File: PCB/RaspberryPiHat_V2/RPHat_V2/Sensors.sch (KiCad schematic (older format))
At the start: 22 parts, among them IC1 TXB0108YZPR2, J15 Conn_01x01, J2 Hall effect connector Right, J3 Halleffect Connector Left, U1 BME680, U2 INA219AxD, U3 ICM-20948, U4 GY-NEO6MV2

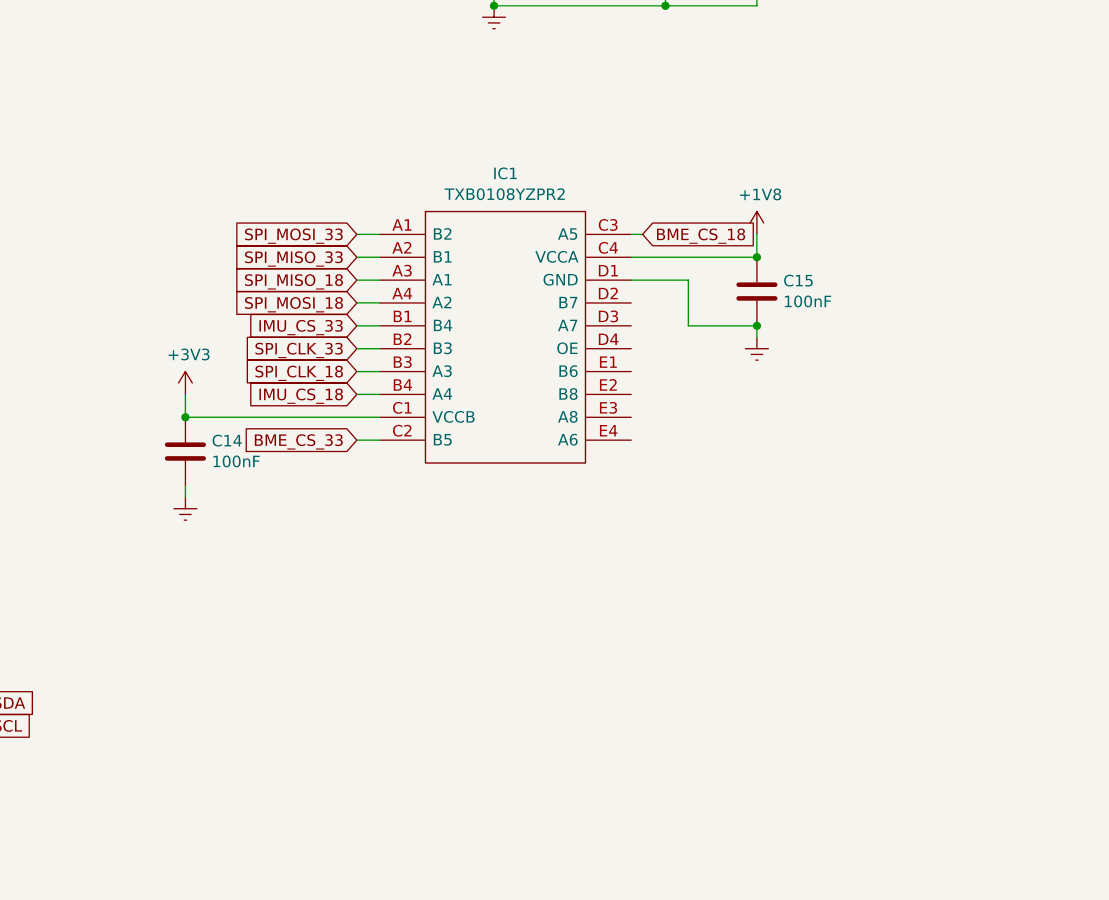
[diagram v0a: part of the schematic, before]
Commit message: started pcb routing
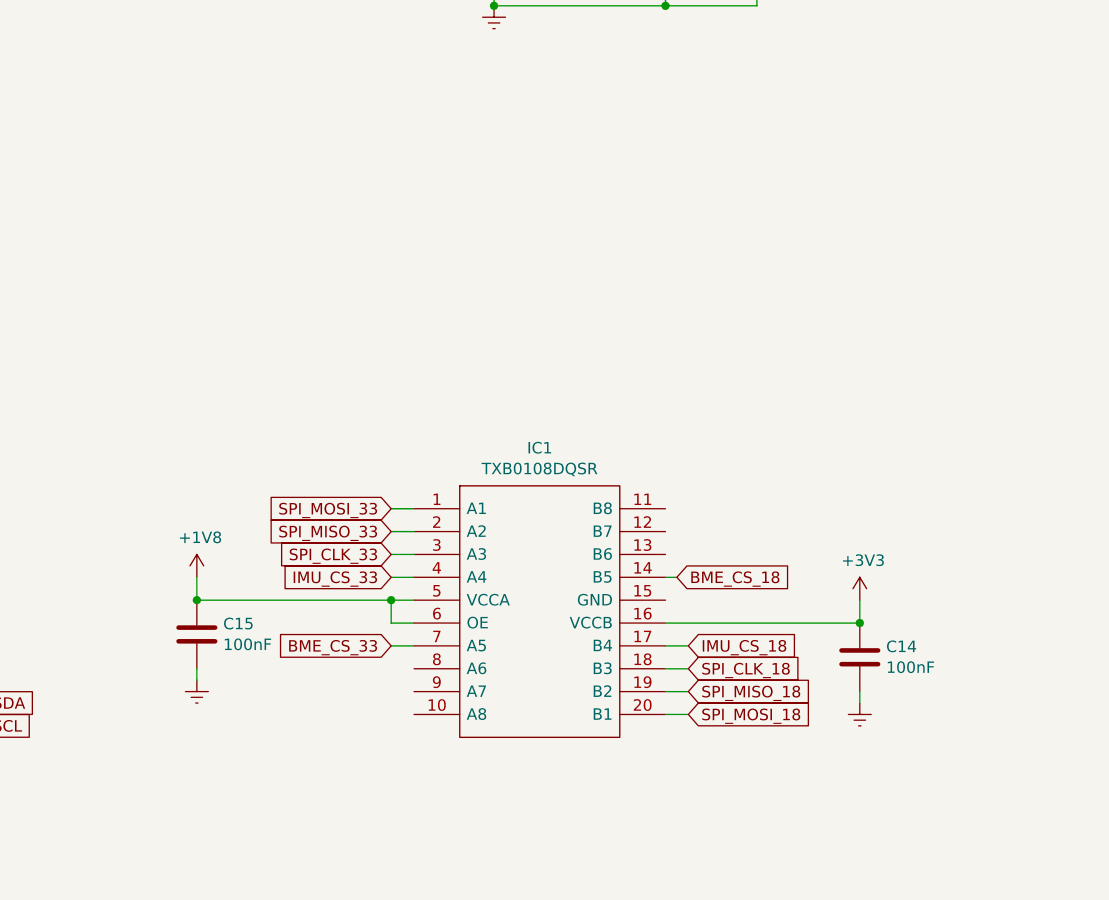
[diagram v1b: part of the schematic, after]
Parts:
- removed IC1: TXB0108YZPR2, TXB0108YZPR2:BGA20C50P4X5_189X239X50, symbol RPHat_V2-rescue:TXB0108YZPR2-TXB0108YZPR2
- added IC1: TXB0108DQSR, User:TXB0108DQSR, symbol User:TXB0108DQSR
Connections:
- net +1V8: now also IC1.5 (VCCA), IC1.6 (OE)
- net +3V3: now also IC1.16 (VCCB)
- net BME_CS_18: now also IC1.14 (B5)
- net BME_CS_33: now also IC1.7 (A5)
- net IMU_CS_18: now also IC1.17 (B4)
- net IMU_CS_33: now also IC1.4 (A4)
- net SPI_CLK_18: now also IC1.18 (B3)
- net SPI_CLK_33: now also IC1.3 (A3)
- net SPI_MISO_18: now also IC1.19 (B2)
- net SPI_MISO_33: now also IC1.2 (A2)
- net SPI_MOSI_18: now also IC1.20 (B1)
- net SPI_MOSI_33: now also IC1.1 (A1)
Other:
- moved on the sheet: C14, C15
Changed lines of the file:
@@
 HE_R_OUTPUT
-$Comp
-L RPHat_V2-rescue:TXB0108YZPR2-TXB0108YZPR2 IC1
-U 1 1 60A9D2C1
-P 6450 3800
-F 0 "IC1" H 7000 4065 50  0000 C CNN
-F 1 "TXB0108YZPR2" H 7000 3974 50  0000 C CNN
-F 2 "TXB0108YZPR2:BGA20C50P4X5_189X239X50" H 7400 3900 50  0001 L CNN
-F 3 "http://www.ti.com/lit/gpn/TXB0108" H 7400 3800 50  0001 L CNN
-F 4 "8-Bit Bidirectional Voltage-Level Shifter with Auto Direction Sensing and +/-15-kV ESD Protect" H 7400 3700 50  0001 L CNN "Description"
-F 5 "0.5" H 7400 3600 50  0001 L CNN "Height"
-F 6 "Texas Instruments" H 7400 3500 50  0001 L CNN "Manufacturer_Name"
-F 7 "TXB0108YZPR2" H 7400 3400 50  0001 L CNN "Manufacturer_Part_Number"
-F 8 "595-TXB0108YZPR2" H 7400 3300 50  0001 L CNN "Mouser Part Number"
-F 9 "https://www.mouser.co.uk/ProductDetail/Texas-Instruments/TXB0108YZPR2?qs=PqoDHHvF64977Sea9xf4wg%3D%3D" H 7400 3200 50  0001 L CNN "Mouser Price/Stock"
-F 10 "TXB0108YZPR2" H 7400 3100 50  0001 L CNN "Arrow Part Number"
-F 11 "https://www.arrow.com/en/products/txb0108yzpr2/texas-instruments" H 7400 3000 50  0001 L CNN "Arrow Price/Stock"
-	1    6450 3800
-	1    0    0    -1
-$EndComp
 $Comp
 L power:+1V8 #PWR0130
 U 1 1 609C23EB
-P 8100 3800
-F 0 "#PWR0130" H 8100 3650 50  0001 C CNN
-F 1 "+1V8" H 8115 3973 50  0000 C CNN
-F 2 "" H 8100 3800 50  0001 C CNN
-F 3 "" H 8100 3800 50  0001 C CNN
-	1    8100 3800
+P 5650 5300
+F 0 "#PWR0130" H 5650 5150 50  0001 C CNN
+F 1 "+1V8" H 5665 5473 50  0000 C CNN
+F 2 "" H 5650 5300 50  0001 C CNN
+F 3 "" H 5650 5300 50  0001 C CNN
+	1    5650 5300
 	1    0    0    -1
 $EndComp
@@
 L power:+3V3 #PWR0131
 U 1 1 609C3DE0
-P 5600 4500
-F 0 "#PWR0131" H 5600 4350 50  0001 C CNN
-F 1 "+3V3" H 5615 4673 50  0000 C CNN
-F 2 "" H 5600 4500 50  0001 C CNN
-F 3 "" H 5600 4500 50  0001 C CNN
-	1    5600 4500
-	1    0    0    -1
-$EndComp
-Wire Wire Line
-	5600 4600 5600 4500
-Wire Wire Line
-	8100 3900 8100 3800
-Wire Wire Line
-	7550 3900 8100 3900
-Text GLabel 6350 4000 0    50   Input ~ 0
-SPI_MISO_18
-Text GLabel 6350 4100 0    50   Input ~ 0
-SPI_MOSI_18
-Text GLabel 6350 4400 0    50   Input ~ 0
+P 8550 5400
+F 0 "#PWR0131" H 8550 5250 50  0001 C CNN
+F 1 "+3V3" H 8565 5573 50  0000 C CNN
+F 2 "" H 8550 5400 50  0001 C CNN
+F 3 "" H 8550 5400 50  0001 C CNN
+	1    8550 5400
+	1    0    0    -1
+$EndComp
+Wire Wire Line
+	5650 5400 5650 5300
+Text GLabel 7800 5700 2    50   Input ~ 0
 SPI_CLK_18
-Text GLabel 6350 4500 0    50   Input ~ 0
+Text GLabel 7800 5600 2    50   Input ~ 0
 IMU_CS_18
-Text GLabel 7600 3800 2    50   Input ~ 0
+Text GLabel 7750 5300 2    50   Input ~ 0
 BME_CS_18
-Text GLabel 6350 3900 0    50   Input ~ 0
+Text GLabel 6500 5100 0    50   Input ~ 0
 SPI_MISO_33
-Text GLabel 6350 3800 0    50   Input ~ 0
+Text GLabel 6500 5000 0    50   Input ~ 0
 SPI_MOSI_33
-Text GLabel 6350 4300 0    50   Input ~ 0
+Text GLabel 6500 5200 0    50   Input ~ 0
 SPI_CLK_33
-Text GLabel 6350 4200 0    50   Input ~ 0
+Text GLabel 6500 5300 0    50   Input ~ 0
 IMU_CS_33
-Text GLabel 6350 4700 0    50   Input ~ 0
+Text GLabel 6500 5600 0    50   Input ~ 0
 BME_CS_33
 Wire Wire Line
-	5600 4600 6450 4600
-Wire Wire Line
-	7600 3800 7550 3800
-Wire Wire Line
-	6350 4000 6450 4000
-Wire Wire Line
-	6350 4100 6450 4100
-Wire Wire Line
-	6350 4400 6450 4400
-Wire Wire Line
-	6350 4500 6450 4500
-Wire Wire Line
-	6350 3800 6450 3800
-Wire Wire Line
-	6350 3900 6450 3900
-Wire Wire Line
-	6350 4200 6450 4200
-Wire Wire Line
-	6350 4300 6450 4300
-Wire Wire Line
-	6350 4700 6450 4700
+	7750 5300 7700 5300
+Wire Wire Line
+	7800 5800 7700 5800
+Wire Wire Line
+	7800 5900 7700 5900
+Wire Wire Line
+	7800 5700 7700 5700
+Wire Wire Line
+	7800 5600 7700 5600
+Wire Wire Line
+	6500 5000 6600 5000
+Wire Wire Line
+	6500 5100 6600 5100
+Wire Wire Line
+	6500 5300 6600 5300
+Wire Wire Line
+	6500 5200 6600 5200
+Wire Wire Line
+	6500 5600 6600 5600
 Text GLabel 4700 5850 2    50   Input ~ 0
 SDA
@@
 L Device:C C14
 U 1 1 60AB39EC
-P 5600 4750
-F 0 "C14" H 5715 4796 50  0000 L CNN
-F 1 "100nF" H 5715 4705 50  0000 L CNN
-F 2 "Capacitor_SMD:C_0603_1608Metric_Pad1.08x0.95mm_HandSolder" H 5638 4600 50  0001 C CNN
-F 3 "~" H 5600 4750 50  0001 C CNN
-	1    5600 4750
+P 8550 5650
+F 0 "C14" H 8665 5696 50  0000 L CNN
+F 1 "100nF" H 8665 5605 50  0000 L CNN
+F 2 "Capacitor_SMD:C_0603_1608Metric_Pad1.08x0.95mm_HandSolder" H 8588 5500 50  0001 C CNN
+F 3 "~" H 8550 5650 50  0001 C CNN
+	1    8550 5650
 	1    0    0    -1
 $EndComp
@@
 L Device:C C15
 U 1 1 60AB76A4
-P 8100 4050
-F 0 "C15" H 8215 4096 50  0000 L CNN
-F 1 "100nF" H 8215 4005 50  0000 L CNN
-F 2 "Capacitor_SMD:C_0603_1608Metric_Pad1.08x0.95mm_HandSolder" H 8138 3900 50  0001 C CNN
-F 3 "~" H 8100 4050 50  0001 C CNN
-	1    8100 4050
+P 5650 5550
+F 0 "C15" H 5765 5596 50  0000 L CNN
+F 1 "100nF" H 5765 5505 50  0000 L CNN
+F 2 "Capacitor_SMD:C_0603_1608Metric_Pad1.08x0.95mm_HandSolder" H 5688 5400 50  0001 C CNN
+F 3 "~" H 5650 5550 50  0001 C CNN
+	1    5650 5550
 	1    0    0    -1
 $EndComp
@@
 L power:GNDREF #PWR01
 U 1 1 60ABB27E
-P 5600 4950
-F 0 "#PWR01" H 5600 4700 50  0001 C CNN
-F 1 "GNDREF" H 5605 4777 50  0001 C CNN
-F 2 "" H 5600 4950 50  0001 C CNN
-F 3 "" H 5600 4950 50  0001 C CNN
-	1    5600 4950
-	1    0    0    -1
-$EndComp
-Wire Wire Line
-	5600 4900 5600 4950
-Connection ~ 8100 3900
+P 8550 5850
+F 0 "#PWR01" H 8550 5600 50  0001 C CNN
+F 1 "GNDREF" H 8555 5677 50  0001 C CNN
+F 2 "" H 8550 5850 50  0001 C CNN
+F 3 "" H 8550 5850 50  0001 C CNN
+	1    8550 5850
+	1    0    0    -1
+$EndComp
+Wire Wire Line
+	8550 5800 8550 5850
 $Comp
 L power:GNDREF #PWR02
 U 1 1 60ACAE6A
-P 8100 4250
-F 0 "#PWR02" H 8100 4000 50  0001 C CNN
-F 1 "GNDREF" H 8105 4077 50  0001 C CNN
-F 2 "" H 8100 4250 50  0001 C CNN
-F 3 "" H 8100 4250 50  0001 C CNN
-	1    8100 4250
-	1    0    0    -1
-$EndComp
-Wire Wire Line
-	8100 4200 8100 4250
-Wire Wire Line
-	7550 4000 7800 4000
-Wire Wire Line
-	7800 4000 7800 4200
-Wire Wire Line
-	7800 4200 8100 4200
-Connection ~ 8100 4200
-Connection ~ 5600 4600
+P 5650 5750
+F 0 "#PWR02" H 5650 5500 50  0001 C CNN
+F 1 "GNDREF" H 5655 5577 50  0001 C CNN
+F 2 "" H 5650 5750 50  0001 C CNN
+F 3 "" H 5650 5750 50  0001 C CNN
+	1    5650 5750
+	1    0    0    -1
+$EndComp
+Wire Wire Line
+	5650 5700 5650 5750
 $Comp
 L Device:R R4
@@
 Wire Wire Line
 	2700 6600 2700 6850
+$Comp
+L User:TXB0108DQSR IC1
+U 1 1 60AA4FBA
+P 6600 5000
+F 0 "IC1" H 7150 5265 50  0000 C CNN
+F 1 "TXB0108DQSR" H 7150 5174 50  0000 C CNN
+F 2 "User:TXB0108DQSR" H 7550 5100 50  0001 L CNN
+F 3 "http://www.ti.com/lit/gpn/txb0108" H 7550 5000 50  0001 L CNN
+F 4 "8-Bit Bidirectional Voltage-Level Shifter with Auto Direction Sensing and +/-15-kV ESD Protect" H 7550 4900 50  0001 L CNN "Description"
+F 5 "0" H 7550 4800 50  0001 L CNN "Height"
+F 6 "Texas Instruments" H 7550 4700 50  0001 L CNN "Manufacturer_Name"
+F 7 "TXB0108DQSR" H 7550 4600 50  0001 L CNN "Manufacturer_Part_Number"
+F 8 "595-TXB0108DQSR" H 7550 4500 50  0001 L CNN "Mouser Part Number"
+F 9 "https://www.mouser.co.uk/ProductDetail/Texas-Instruments/TXB0108DQSR?qs=EuM%2FBx4ov4SMZCOlCh%2FWxA%3D%3D" H 7550 4400 50  0001 L CNN "Mouser Price/Stock"
+F 10 "TXB0108DQSR" H 7550 4300 50  0001 L CNN "Arrow Part Number"
+F 11 "https://www.arrow.com/en/products/txb0108dqsr/texas-instruments" H 7550 4200 50  0001 L CNN "Arrow Price/Stock"
+	1    6600 5000
+	1    0    0    -1
+$EndComp
+Wire Wire Line
+	8550 5500 8550 5400
+Connection ~ 8550 5500
+Text GLabel 7800 5900 2    50   Input ~ 0
+SPI_MOSI_18
+Text GLabel 7800 5800 2    50   Input ~ 0
+SPI_MISO_18
+Wire Wire Line
+	7700 5500 8550 5500
+Wire Wire Line
+	6600 5500 6500 5500
+Wire Wire Line
+	6500 5500 6500 5400
+Wire Wire Line
+	6500 5400 6600 5400
+Wire Wire Line
+	6500 5400 5650 5400
+Connection ~ 6500 5400
+Connection ~ 5650 5400
 $EndSCHEMATC
